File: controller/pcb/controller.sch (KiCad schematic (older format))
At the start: 59 parts, among them J1 POWER, J2 10K POT, Q1 2N2222, Q12 TIP41, Q13 TIP41, Q14 2N2907, Q15 2N2222, Q2 TIP42, Q3 TIP42, Q4 2N2222, Q5 2N2222, U1 LM78M05_TO220, U2 PIC12F1501-ISN, U3 74HC595

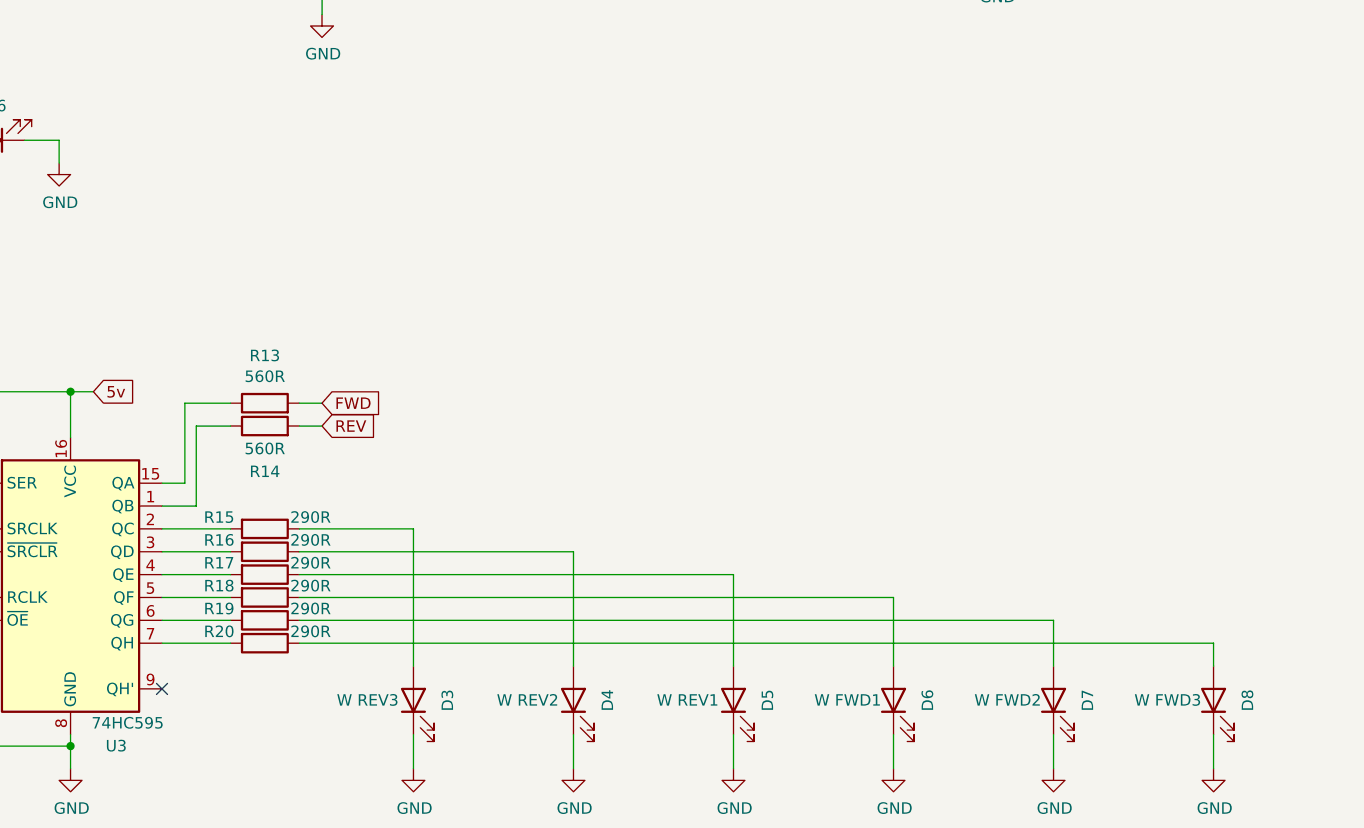
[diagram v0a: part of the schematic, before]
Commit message: Further firmware tweaks.
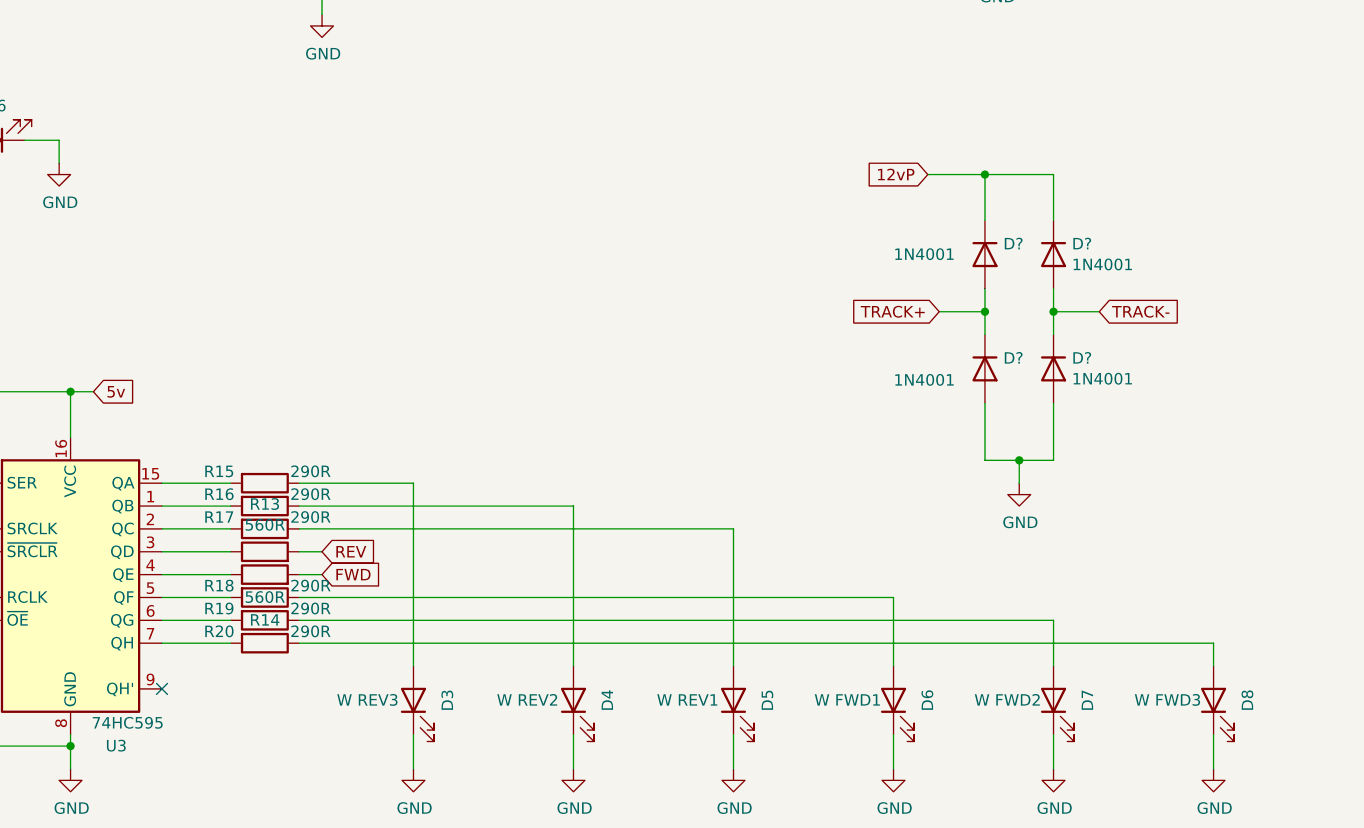
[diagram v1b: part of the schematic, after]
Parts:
- added D? (x4): 1N4001, symbol Device:D
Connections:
- net 12vP: now also D?.1 (K), D?.1 (K)
- net FWD: now also R14.2; no longer R13.2
- net GND: now also D?.2 (A), D?.2 (A)
- net REV: now also R13.2; no longer R14.2
- net TRACK+: now also D?.1 (K), D?.2 (A)
- net TRACK-: now also D?.1 (K), D?.2 (A)
- net at R15.2: now also U3.15 (QA); no longer U3.2 (QC)
- net at R16.2: now also U3.1 (QB); no longer U3.3 (QD)
- net at R17.2: now also U3.2 (QC); no longer U3.4 (QE)
- net at R14.1: now also U3.4 (QE); no longer U3.1 (QB)
- net at R13.1: now also U3.3 (QD); no longer U3.15 (QA)
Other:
- moved on the sheet: R13, R14, R15, R16, R17
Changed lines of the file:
@@
 	1    0    0    -1
 $EndComp
-Text GLabel 6350 4000 2    50   Input ~ 0
+Text GLabel 6350 4750 2    50   Input ~ 0
 FWD
-Text GLabel 6350 4100 2    50   Input ~ 0
+Text GLabel 6350 4650 2    50   Input ~ 0
 REV
 $Comp
@@
 L Device:R R14
 U 1 1 5EF1835E
-P 6100 4100
-F 0 "R14" V 5900 4100 50  0000 C CNN
-F 1 "560R" V 6000 4100 50  0000 C CNN
-F 2 "Resistors_THT:R_Axial_DIN0411_L9.9mm_D3.6mm_P12.70mm_Horizontal" V 6030 4100 50  0001 C CNN
-F 3 "~" H 6100 4100 50  0001 C CNN
-	1    6100 4100
+P 6100 4750
+F 0 "R14" V 5900 4750 50  0000 C CNN
+F 1 "560R" V 6000 4750 50  0000 C CNN
+F 2 "Resistors_THT:R_Axial_DIN0411_L9.9mm_D3.6mm_P12.70mm_Horizontal" V 6030 4750 50  0001 C CNN
+F 3 "~" H 6100 4750 50  0001 C CNN
+	1    6100 4750
 	0    -1   -1   0
 $EndComp
@@
 L Device:R R13
 U 1 1 5EF1860D
-P 6100 4000
-F 0 "R13" V 6307 4000 50  0000 C CNN
-F 1 "560R" V 6216 4000 50  0000 C CNN
-F 2 "Resistors_THT:R_Axial_DIN0411_L9.9mm_D3.6mm_P12.70mm_Horizontal" V 6030 4000 50  0001 C CNN
-F 3 "~" H 6100 4000 50  0001 C CNN
-	1    6100 4000
+P 6100 4650
+F 0 "R13" V 6307 4650 50  0000 C CNN
+F 1 "560R" V 6216 4650 50  0000 C CNN
+F 2 "Resistors_THT:R_Axial_DIN0411_L9.9mm_D3.6mm_P12.70mm_Horizontal" V 6030 4650 50  0001 C CNN
+F 3 "~" H 6100 4650 50  0001 C CNN
+	1    6100 4650
 	0    -1   -1   0
 $EndComp
@@
 	5250 5450 5250 5500
 Wire Wire Line
-	6350 4000 6250 4000
-Wire Wire Line
-	6250 4100 6350 4100
-Wire Wire Line
-	5950 4000 5750 4000
-Wire Wire Line
-	5750 4000 5750 4350
-Wire Wire Line
-	5750 4350 5650 4350
-Wire Wire Line
-	5950 4100 5800 4100
-Wire Wire Line
-	5800 4100 5800 4450
-Wire Wire Line
-	5800 4450 5650 4450
+	6350 4650 6250 4650
+Wire Wire Line
+	6250 4750 6350 4750
 Text GLabel 4700 4350 0    50   Input ~ 0
 DATA
@@
 L Device:R R15
 U 1 1 5ECDE1CF
-P 6100 4550
-F 0 "R15" V 6050 4350 50  0000 C CNN
-F 1 "290R" V 6050 4750 50  0000 C CNN
-F 2 "Resistors_THT:R_Axial_DIN0411_L9.9mm_D3.6mm_P12.70mm_Horizontal" V 6030 4550 50  0001 C CNN
-F 3 "~" H 6100 4550 50  0001 C CNN
-	1    6100 4550
-	0    1    1    0
-$EndComp
-Wire Wire Line
-	5650 4550 5950 4550
-Wire Wire Line
-	6250 4550 6750 4550
+P 6100 4350
+F 0 "R15" V 6050 4150 50  0000 C CNN
+F 1 "290R" V 6050 4550 50  0000 C CNN
+F 2 "Resistors_THT:R_Axial_DIN0411_L9.9mm_D3.6mm_P12.70mm_Horizontal" V 6030 4350 50  0001 C CNN
+F 3 "~" H 6100 4350 50  0001 C CNN
+	1    6100 4350
+	0    1    1    0
+$EndComp
+Wire Wire Line
+	6250 4350 6750 4350
 $Comp
 L Device:LED D3
@@
 L Device:R R16
 U 1 1 5ED4926F
-P 6100 4650
-F 0 "R16" V 6050 4450 50  0000 C CNN
-F 1 "290R" V 6050 4850 50  0000 C CNN
-F 2 "Resistors_THT:R_Axial_DIN0411_L9.9mm_D3.6mm_P12.70mm_Horizontal" V 6030 4650 50  0001 C CNN
-F 3 "~" H 6100 4650 50  0001 C CNN
-	1    6100 4650
+P 6100 4450
+F 0 "R16" V 6050 4250 50  0000 C CNN
+F 1 "290R" V 6050 4650 50  0000 C CNN
+F 2 "Resistors_THT:R_Axial_DIN0411_L9.9mm_D3.6mm_P12.70mm_Horizontal" V 6030 4450 50  0001 C CNN
+F 3 "~" H 6100 4450 50  0001 C CNN
+	1    6100 4450
 	0    1    1    0
 $EndComp
@@
 L Device:R R17
 U 1 1 5ED49375
-P 6100 4750
-F 0 "R17" V 6050 4550 50  0000 C CNN
-F 1 "290R" V 6050 4950 50  0000 C CNN
-F 2 "Resistors_THT:R_Axial_DIN0411_L9.9mm_D3.6mm_P12.70mm_Horizontal" V 6030 4750 50  0001 C CNN
-F 3 "~" H 6100 4750 50  0001 C CNN
-	1    6100 4750
+P 6100 4550
+F 0 "R17" V 6050 4350 50  0000 C CNN
+F 1 "290R" V 6050 4750 50  0000 C CNN
+F 2 "Resistors_THT:R_Axial_DIN0411_L9.9mm_D3.6mm_P12.70mm_Horizontal" V 6030 4550 50  0001 C CNN
+F 3 "~" H 6100 4550 50  0001 C CNN
+	1    6100 4550
 	0    1    1    0
 $EndComp
@@
 $EndComp
 Wire Wire Line
-	5650 4650 5950 4650
-Wire Wire Line
-	5650 4750 5950 4750
-Wire Wire Line
 	5650 4850 5950 4850
 Wire Wire Line
@@
 	5650 5050 5950 5050
 Wire Wire Line
-	6250 4650 7450 4650
-Wire Wire Line
-	6250 4750 8150 4750
+	6250 4450 7450 4450
+Wire Wire Line
+	6250 4550 8150 4550
 Wire Wire Line
 	6250 4850 8850 4850
@@
 	8850 4850 8850 5150
 Wire Wire Line
-	8150 4750 8150 5150
-Wire Wire Line
-	7450 4650 7450 5150
-Wire Wire Line
-	6750 4550 6750 5150
+	8150 4550 8150 5150
+Wire Wire Line
+	7450 4450 7450 5150
+Wire Wire Line
+	6750 4350 6750 5150
+$Comp
+L Device:D D?
+U 1 1 5EF8C3FB
+P 9250 3350
+F 0 "D?" V 9204 3430 50  0000 L CNN
+F 1 "1N4001" V 9250 2950 50  0000 L CNN
+F 2 "" H 9250 3350 50  0001 C CNN
+F 3 "~" H 9250 3350 50  0001 C CNN
+	1    9250 3350
+	0    1    1    0
+$EndComp
+Text GLabel 9000 3000 0    50   Input ~ 0
+12vP
+Text GLabel 9050 3600 0    50   Input ~ 0
+TRACK+
+Text GLabel 9750 3600 2    50   Input ~ 0
+TRACK-
+$Comp
+L Device:D D?
+U 1 1 5EF8DBEF
+P 9250 3850
+F 0 "D?" V 9204 3930 50  0000 L CNN
+F 1 "1N4001" V 9300 3450 50  0000 L CNN
+F 2 "" H 9250 3850 50  0001 C CNN
+F 3 "~" H 9250 3850 50  0001 C CNN
+	1    9250 3850
+	0    1    1    0
+$EndComp
+$Comp
+L Device:D D?
+U 1 1 5EF8DD5D
+P 9550 3350
+F 0 "D?" V 9504 3430 50  0000 L CNN
+F 1 "1N4001" V 9595 3430 50  0000 L CNN
+F 2 "" H 9550 3350 50  0001 C CNN
+F 3 "~" H 9550 3350 50  0001 C CNN
+	1    9550 3350
+	0    1    1    0
+$EndComp
+$Comp
+L Device:D D?
+U 1 1 5EF8DE71
+P 9550 3850
+F 0 "D?" V 9504 3930 50  0000 L CNN
+F 1 "1N4001" V 9595 3930 50  0000 L CNN
+F 2 "" H 9550 3850 50  0001 C CNN
+F 3 "~" H 9550 3850 50  0001 C CNN
+	1    9550 3850
+	0    1    1    0
+$EndComp
+Wire Wire Line
+	9000 3000 9250 3000
+Wire Wire Line
+	9250 3000 9250 3200
+Wire Wire Line
+	9250 3000 9550 3000
+Wire Wire Line
+	9550 3000 9550 3200
+Wire Wire Line
+	9250 3500 9250 3600
+Wire Wire Line
+	9550 3500 9550 3600
+Wire Wire Line
+	9250 4000 9250 4250
+Wire Wire Line
+	9550 4000 9550 4250
+Wire Wire Line
+	9550 4250 9400 4250
+Wire Wire Line
+	9050 3600 9250 3600
+Connection ~ 9250 3600
+Wire Wire Line
+	9250 3600 9250 3700
+Wire Wire Line
+	9750 3600 9550 3600
+Connection ~ 9550 3600
+Wire Wire Line
+	9550 3600 9550 3700
+$Comp
+L power:GND #PWR?
+U 1 1 5EFD4272
+P 9400 4350
+F 0 "#PWR?" H 9400 4100 50  0001 C CNN
+F 1 "GND" H 9405 4177 50  0000 C CNN
+F 2 "" H 9400 4350 50  0001 C CNN
+F 3 "" H 9400 4350 50  0001 C CNN
+	1    9400 4350
+	1    0    0    -1
+$EndComp
+Connection ~ 9250 3000
+Wire Wire Line
+	9400 4350 9400 4250
+Connection ~ 9400 4250
+Wire Wire Line
+	9400 4250 9250 4250
+Wire Wire Line
+	5650 4350 5950 4350
+Wire Wire Line
+	5650 4450 5950 4450
+Wire Wire Line
+	5650 4550 5950 4550
+Wire Wire Line
+	5650 4650 5950 4650
+Wire Wire Line
+	5650 4750 5950 4750
 $EndSCHEMATC
